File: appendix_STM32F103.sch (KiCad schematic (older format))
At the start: 41 parts, among them J201 Micro_SD_Card_Det, J202 Conn_02x05_Odd_Even, J203 Conn_02x20_Odd_Even, J204 Conn_ARM_JTAG_SWD_10, SW201 SW_Push, U201 STM32F103ZETx, U202 NTS0104PW-Q100J, U203 NTS0104PW-Q100J, X201 SG-210STF

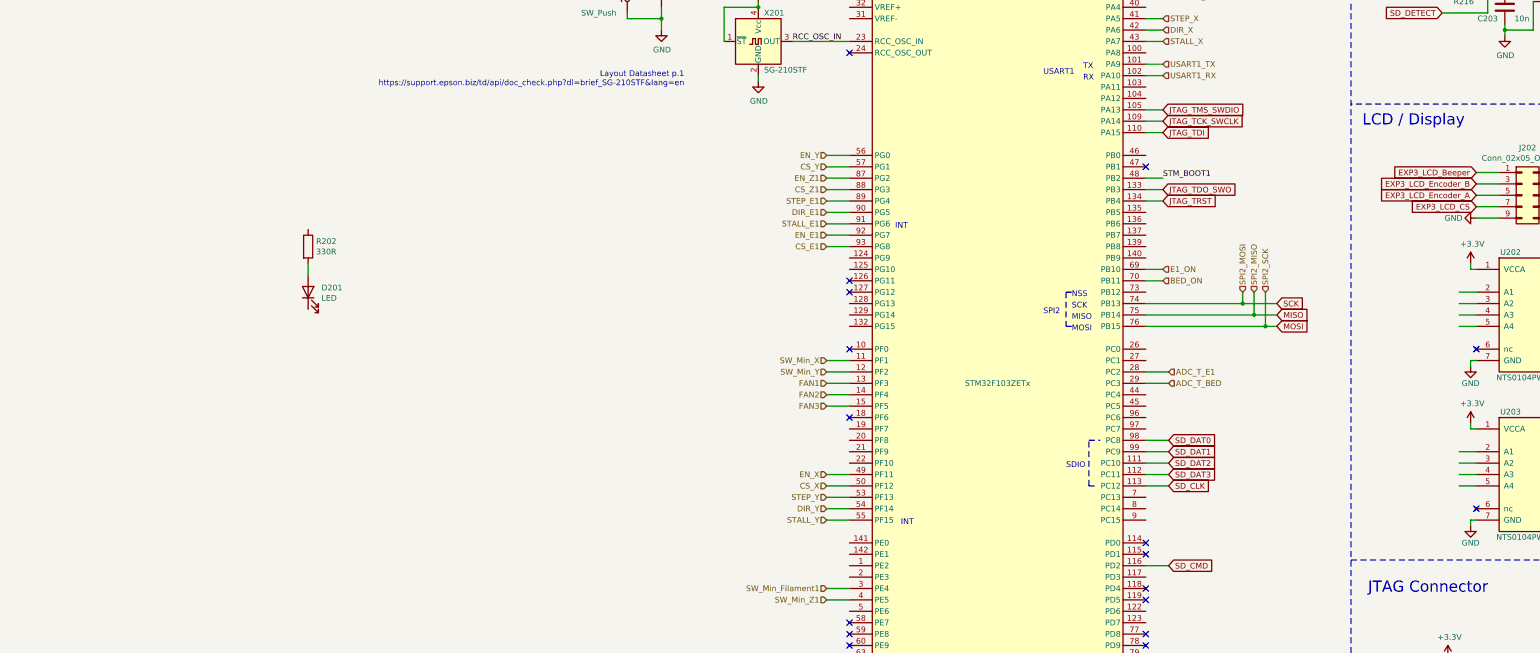
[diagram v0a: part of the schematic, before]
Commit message: user LED + fixes in Layout
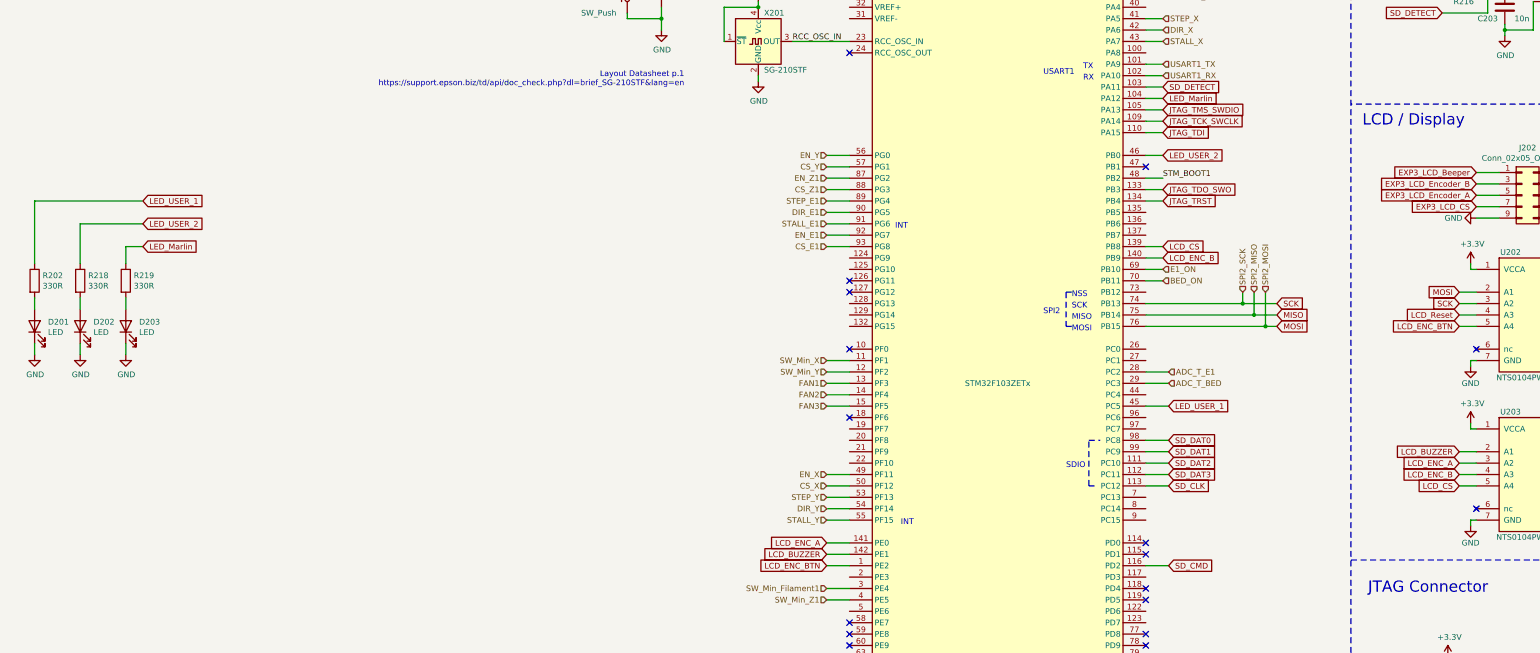
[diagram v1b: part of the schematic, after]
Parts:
- added D202, D203: LED, LED_SMD:LED_0805_2012Metric, symbol Device:LED
- added R218, R219: 330R, Resistors_SMD:R_0603, symbol Device:R
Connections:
- net GND: now also D201.1 (K), D202.1 (K), D203.1 (K)
- net MOSI: now also U202.2 (A1)
- net SCK: now also U202.3 (A2)
- net SD_DETECT: now also U201.103 (PA11)
- net LCD_ENC_BTN: now reaches U201.1 (PE2)
- net LCD_ENC_BTN: now also U202.5 (A4)
- net LED_Marlin: now reaches U201.104 (PA12)
- net LED_Marlin: now also R219.1
- net LCD_CS: now reaches U201.139 (PB8)
- net LCD_CS: now also U203.5 (A4)
- net LCD_ENC_B: now reaches U201.140 (PB9)
- net LCD_ENC_B: now also U203.4 (A3)
- net LCD_ENC_A: now reaches U201.141 (PE0)
- net LCD_ENC_A: now also U203.3 (A2)
- net LCD_BUZZER: now reaches U201.142 (PE1)
- net LCD_BUZZER: now also U203.2 (A1)
- net LED_USER_1: now reaches U201.45 (PC5)
- net LED_USER_1: now also R202.1
- net LED_USER_2: now reaches U201.46 (PB0)
- net LED_USER_2: now also R218.1
- net LCD_Reset: now reaches U202.4 (A3)
- new net: D202.2 (A), R218.2
- new net: D203.2 (A), R219.2
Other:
- moved on the sheet: D201, R202
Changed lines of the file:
@@
 Text HLabel 10850 2200 2    50   Input ~ 0
 USART2_RX
-Text HLabel 11750 4800 1    50   Input ~ 0
+Text HLabel 11550 4800 1    50   Input ~ 0
 SPI2_SCK
 Text HLabel 11650 4800 1    50   Input ~ 0
 SPI2_MISO
-Text HLabel 11550 4800 1    50   Input ~ 0
+Text HLabel 11750 4800 1    50   Input ~ 0
 SPI2_MOSI
 Text HLabel 7900 3600 0    50   Input ~ 0
@@
 L Device:R R202
 U 1 1 5CDABFCE
-P 3350 4400
-F 0 "R202" H 3420 4446 50  0000 L CNN
-F 1 "330R" H 3420 4355 50  0000 L CNN
-F 2 "Resistors_SMD:R_0603" V 3280 4400 50  0001 C CNN
-F 3 "~" H 3350 4400 50  0001 C CNN
-	1    3350 4400
+P 950 4700
+F 0 "R202" H 1020 4746 50  0000 L CNN
+F 1 "330R" H 1020 4655 50  0000 L CNN
+F 2 "Resistors_SMD:R_0603" V 880 4700 50  0001 C CNN
+F 3 "~" H 950 4700 50  0001 C CNN
+	1    950  4700
 	1    0    0    -1
 $EndComp
@@
 L Device:LED D201
 U 1 1 5CDABFD4
-P 3350 4800
-F 0 "D201" V 3389 4683 50  0000 R CNN
-F 1 "LED" V 3298 4683 50  0000 R CNN
-F 2 "LED_SMD:LED_0805_2012Metric" H 3350 4800 50  0001 C CNN
-F 3 "~" H 3350 4800 50  0001 C CNN
-	1    3350 4800
+P 950 5100
+F 0 "D201" V 989 4983 50  0000 R CNN
+F 1 "LED" V 898 4983 50  0000 R CNN
+F 2 "LED_SMD:LED_0805_2012Metric" H 950 5100 50  0001 C CNN
+F 3 "~" H 950 5100 50  0001 C CNN
+	1    950  5100
 	0    -1   -1   0
 $EndComp
 Wire Wire Line
-	3350 4550 3350 4650
+	950  4850 950  4950
 $Comp
 L Connector_Generic:Conn_02x20_Odd_Even J203
@@
 Wire Wire Line
 	8100 5500 7900 5500
+Text GLabel 13450 4900 0    50   Input ~ 0
+SCK
+Text GLabel 13450 4800 0    50   Input ~ 0
+MOSI
+Text GLabel 13450 5000 0    50   Input ~ 0
+LCD_Reset
+Text GLabel 13450 5100 0    50   Input ~ 0
+LCD_ENC_BTN
+Text GLabel 13450 6200 0    50   Input ~ 0
+LCD_BUZZER
+Text GLabel 13450 6300 0    50   Input ~ 0
+LCD_ENC_A
+Text GLabel 13450 6400 0    50   Input ~ 0
+LCD_ENC_B
+Text GLabel 13450 6500 0    50   Input ~ 0
+LCD_CS
+Text GLabel 7900 7200 0    50   Input ~ 0
+LCD_ENC_BTN
+Wire Wire Line
+	8100 7200 7900 7200
+Text GLabel 7900 7100 0    50   Input ~ 0
+LCD_BUZZER
+Text GLabel 7900 7000 0    50   Input ~ 0
+LCD_ENC_A
+Text GLabel 10850 4500 2    50   Input ~ 0
+LCD_ENC_B
+Text GLabel 10850 4400 2    50   Input ~ 0
+LCD_CS
+Wire Wire Line
+	10850 4400 10700 4400
+Wire Wire Line
+	10700 4500 10850 4500
+Wire Wire Line
+	7900 7000 8100 7000
+Wire Wire Line
+	8100 7100 7900 7100
+Text GLabel 10850 3000 2    50   Input ~ 0
+SD_DETECT
+Wire Wire Line
+	10850 3000 10700 3000
+$Comp
+L Device:R R218
+U 1 1 5CEF3625
+P 1350 4700
+F 0 "R218" H 1420 4746 50  0000 L CNN
+F 1 "330R" H 1420 4655 50  0000 L CNN
+F 2 "Resistors_SMD:R_0603" V 1280 4700 50  0001 C CNN
+F 3 "~" H 1350 4700 50  0001 C CNN
+	1    1350 4700
+	1    0    0    -1
+$EndComp
+$Comp
+L Device:LED D202
+U 1 1 5CEF362F
+P 1350 5100
+F 0 "D202" V 1389 4983 50  0000 R CNN
+F 1 "LED" V 1298 4983 50  0000 R CNN
+F 2 "LED_SMD:LED_0805_2012Metric" H 1350 5100 50  0001 C CNN
+F 3 "~" H 1350 5100 50  0001 C CNN
+	1    1350 5100
+	0    -1   -1   0
+$EndComp
+Wire Wire Line
+	1350 4850 1350 4950
+$Comp
+L Device:R R219
+U 1 1 5CF13CB8
+P 1750 4700
+F 0 "R219" H 1820 4746 50  0000 L CNN
+F 1 "330R" H 1820 4655 50  0000 L CNN
+F 2 "Resistors_SMD:R_0603" V 1680 4700 50  0001 C CNN
+F 3 "~" H 1750 4700 50  0001 C CNN
+	1    1750 4700
+	1    0    0    -1
+$EndComp
+$Comp
+L Device:LED D203
+U 1 1 5CF13CC2
+P 1750 5100
+F 0 "D203" V 1789 4983 50  0000 R CNN
+F 1 "LED" V 1698 4983 50  0000 R CNN
+F 2 "LED_SMD:LED_0805_2012Metric" H 1750 5100 50  0001 C CNN
+F 3 "~" H 1750 5100 50  0001 C CNN
+	1    1750 5100
+	0    -1   -1   0
+$EndComp
+Wire Wire Line
+	1750 4850 1750 4950
+$Comp
+L power:GND #PWR0194
+U 1 1 5CF54C9D
+P 950 5350
+F 0 "#PWR0194" H 950 5100 50  0001 C CNN
+F 1 "GND" H 955 5177 50  0000 C CNN
+F 2 "" H 950 5350 50  0001 C CNN
+F 3 "" H 950 5350 50  0001 C CNN
+	1    950  5350
+	1    0    0    -1
+$EndComp
+Wire Wire Line
+	950  5350 950  5250
+$Comp
+L power:GND #PWR0198
+U 1 1 5CF75AD3
+P 1350 5350
+F 0 "#PWR0198" H 1350 5100 50  0001 C CNN
+F 1 "GND" H 1355 5177 50  0000 C CNN
+F 2 "" H 1350 5350 50  0001 C CNN
+F 3 "" H 1350 5350 50  0001 C CNN
+	1    1350 5350
+	1    0    0    -1
+$EndComp
+Wire Wire Line
+	1350 5350 1350 5250
+$Comp
+L power:GND #PWR0199
+U 1 1 5CF96A3E
+P 1750 5350
+F 0 "#PWR0199" H 1750 5100 50  0001 C CNN
+F 1 "GND" H 1755 5177 50  0000 C CNN
+F 2 "" H 1750 5350 50  0001 C CNN
+F 3 "" H 1750 5350 50  0001 C CNN
+	1    1750 5350
+	1    0    0    -1
+$EndComp
+Wire Wire Line
+	1750 5350 1750 5250
+Text GLabel 1900 4400 2    50   Input ~ 0
+LED_Marlin
+Wire Wire Line
+	1900 4400 1750 4400
+Wire Wire Line
+	1750 4400 1750 4550
+Text GLabel 1900 4200 2    50   Input ~ 0
+LED_USER_2
+Text GLabel 1900 4000 2    50   Input ~ 0
+LED_USER_1
+Wire Wire Line
+	1900 4200 1350 4200
+Wire Wire Line
+	1350 4200 1350 4550
+Wire Wire Line
+	1900 4000 950  4000
+Wire Wire Line
+	950  4000 950  4550
+Text GLabel 10900 5800 2    50   Input ~ 0
+LED_USER_1
+Wire Wire Line
+	10900 5800 10700 5800
+Text GLabel 10850 3600 2    50   Input ~ 0
+LED_USER_2
+Wire Wire Line
+	10850 3600 10700 3600
+Text GLabel 10850 3100 2    50   Input ~ 0
+LED_Marlin
+Wire Wire Line
+	10850 3100 10700 3100
 $EndSCHEMATC
